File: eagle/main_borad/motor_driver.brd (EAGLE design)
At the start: 43.2 x 38.1 mm, 17 parts, among them IC1 MEGA8-AI

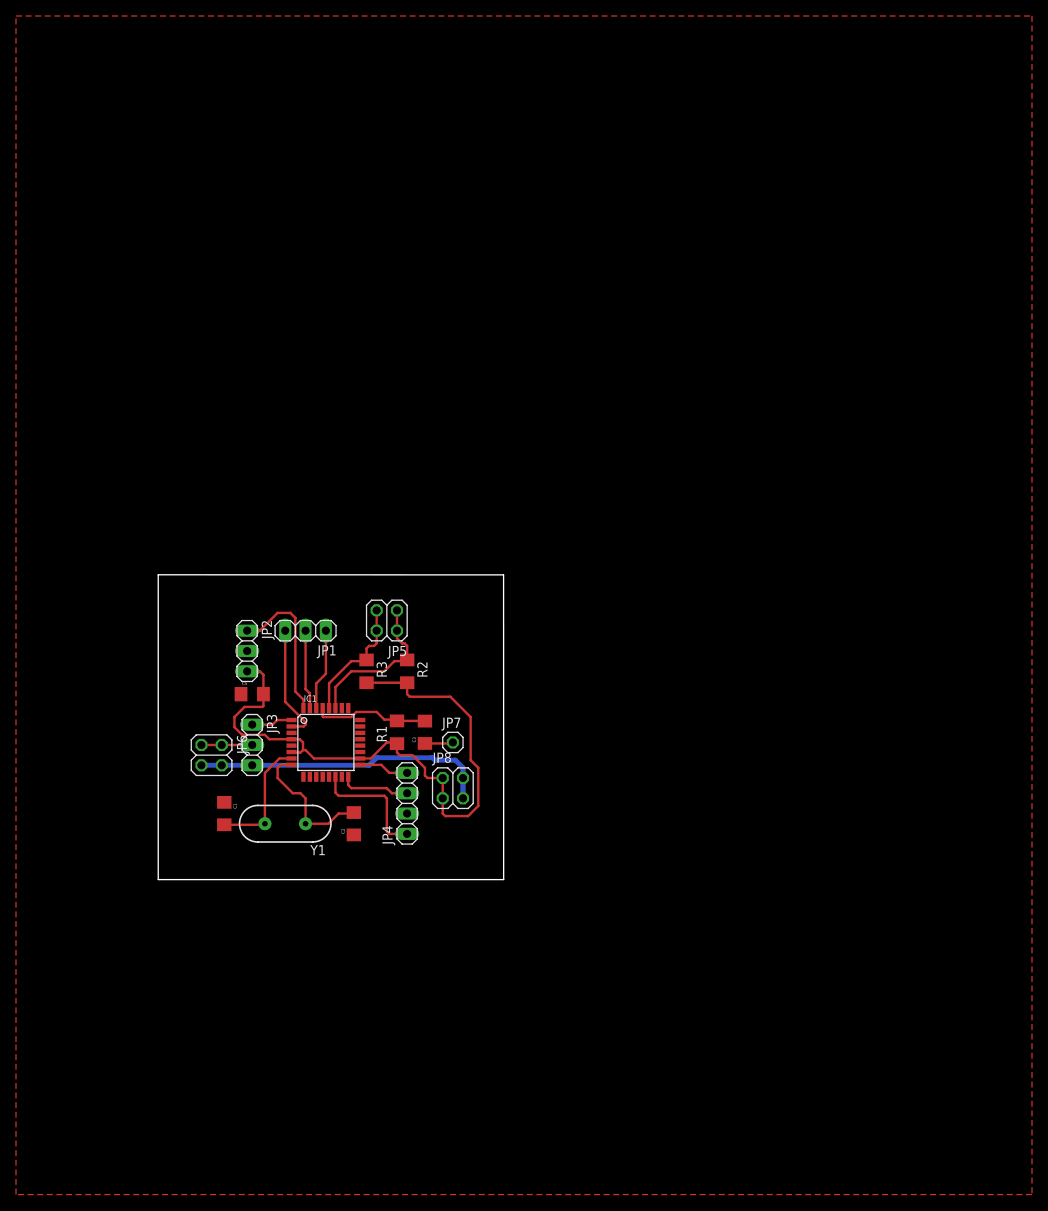
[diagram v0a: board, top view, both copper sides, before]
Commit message: PCB ver. 4.0
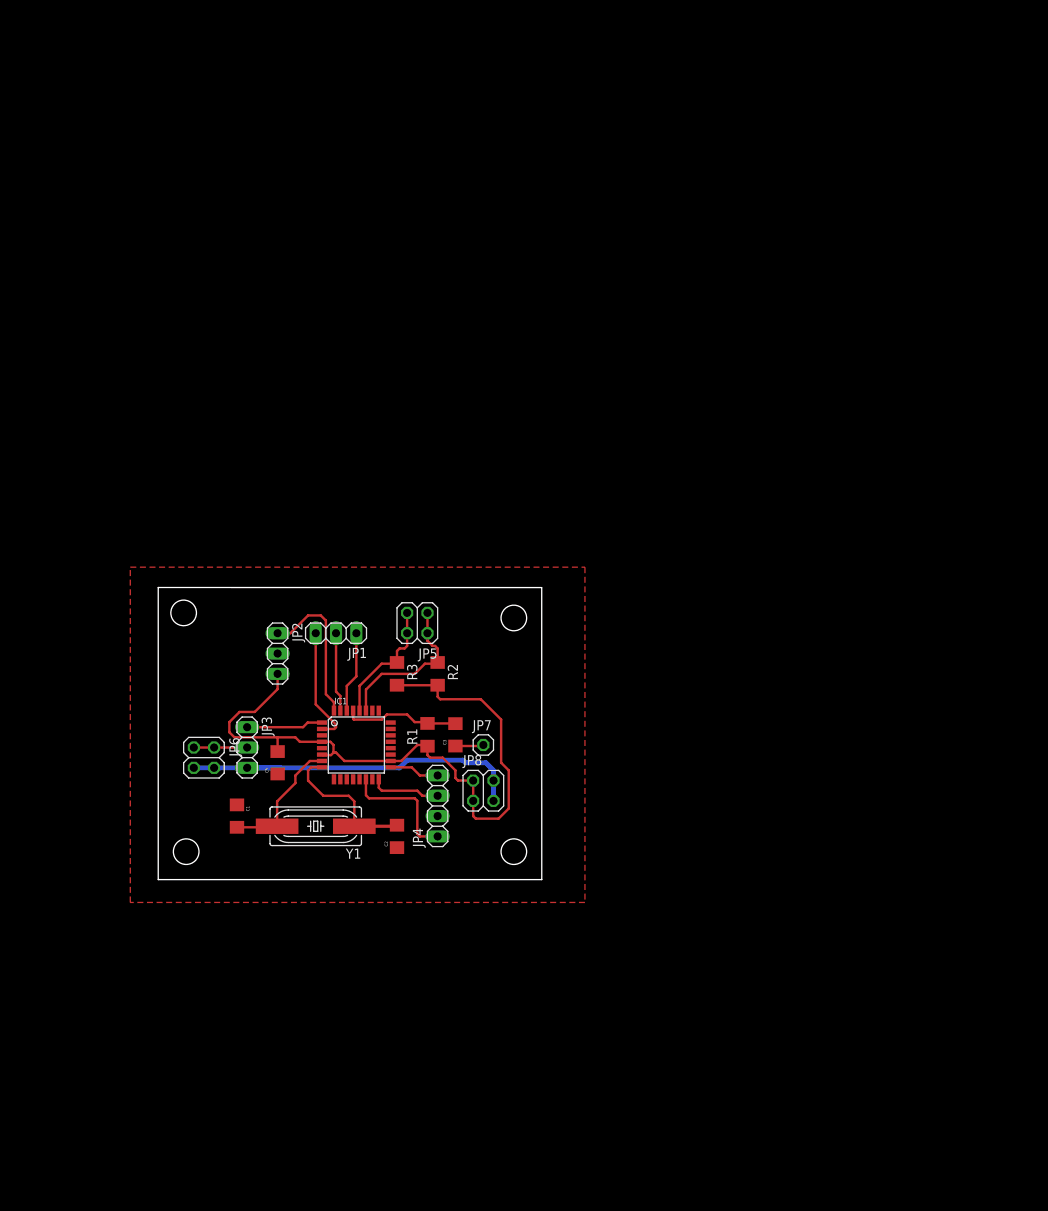
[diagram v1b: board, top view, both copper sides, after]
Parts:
- Y1: device SparkFun-FreqCtrl:HC49US -> SparkFun-FreqCtrl:HC49UP
- moved C5 9.14 mm to (14.9, 14.6), turned to 90 degrees
- moved C2 5.63 mm to (29.8, 5.40)
- moved C3 3.82 mm to (37.1, 18.1)
- moved IC1 3.82 mm to (24.8, 16.8)
- moved JP1 3.82 mm to (22.2, 30.8)
- moved JP7 3.82 mm to (40.6, 16.8)
- moved JP8 3.82 mm to (40.6, 11.1)
- moved R1 3.82 mm to (33.7, 18.1)
- moved JP2 3.82 mm to (14.9, 28.3)
- moved JP4 3.82 mm to (34.9, 9.21)
- moved JP5 3.82 mm to (32.4, 32.1)
- moved R2 3.82 mm to (34.9, 25.7)
- moved R3 3.82 mm to (29.8, 25.7)
- moved Y1 3.82 mm to (19.7, 6.67)
- moved C1 1.62 mm to (9.84, 7.94)
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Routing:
- net GND: track 37.1 -> 46.3 mm
- net N$3: track 15.6 -> 20.7 mm
- net INT1: track 5.15 -> 9.60 mm
- net VCC: track 90.1 -> 94.1 mm
- net N$2: track 17.5 -> 18.6 mm
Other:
- board size 43.2 x 38.1 mm -> 47.9 x 36.5 mm
